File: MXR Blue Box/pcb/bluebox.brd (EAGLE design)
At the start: 59 x 87.8 mm, 20 parts, among them IC2 TL074, J1 POWER_JACK, X1 2510-

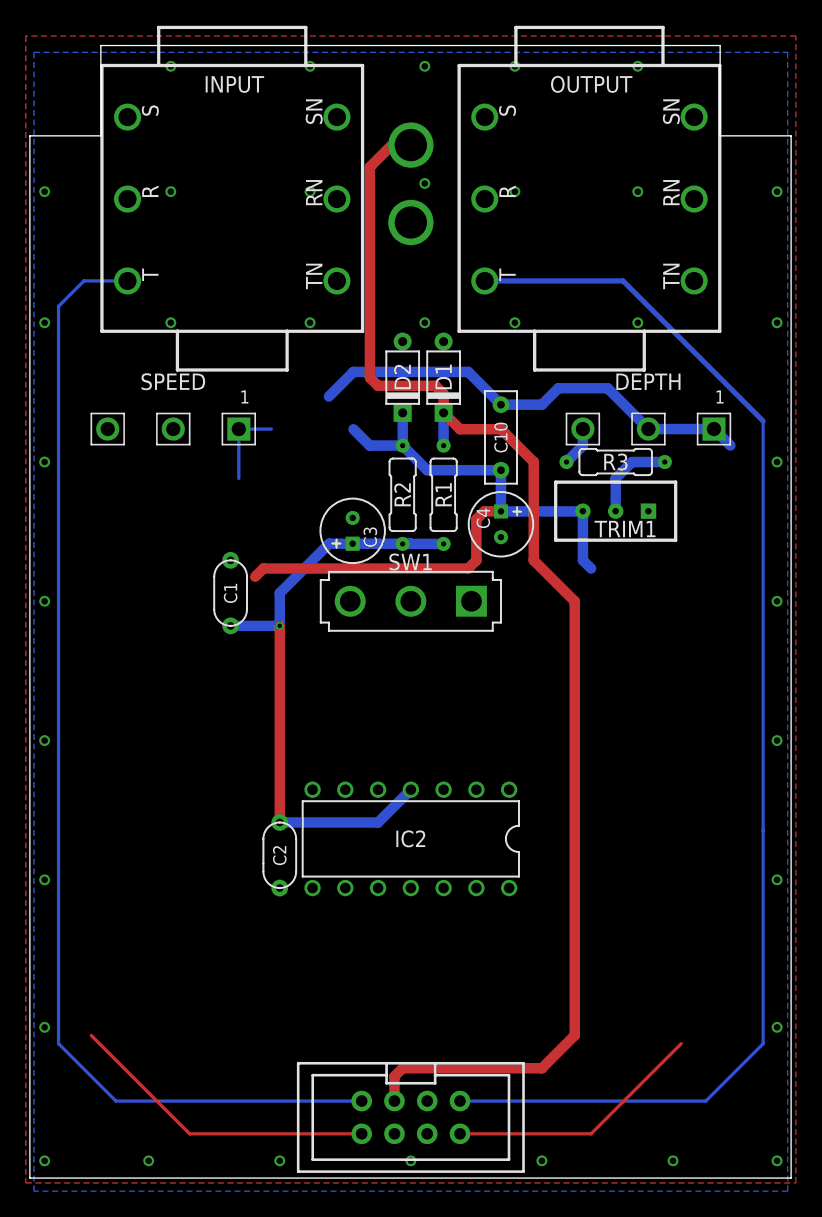
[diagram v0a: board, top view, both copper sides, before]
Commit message: 20171216
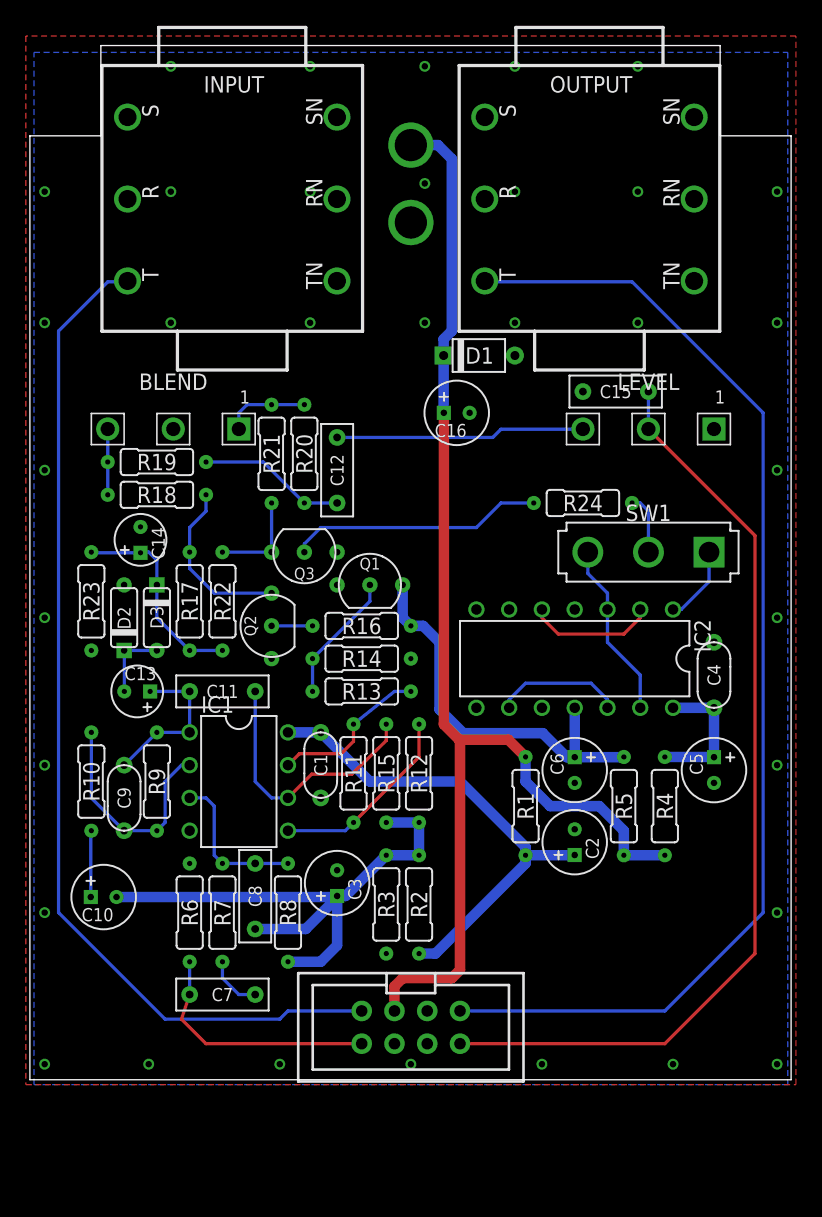
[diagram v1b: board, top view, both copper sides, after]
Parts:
- removed TRIM1: 250k, pedals-potentiometers:RTRIM3296W
- added C11, C12: 47n, pedals-capacitors-film:BOX_SMALL
- added C13, C14: 1u, pedals-capacitors-elec:040_020
- added C15: 6.8n, pedals-capacitors-film:BOX_SMALL
- added C16, C5, C6: 100u, pedals-capacitors-elec:050_020
- added C7: 10n, pedals-capacitors-film:BOX_SMALL
- added C8: 1n, pedals-capacitors-film:BOX_SMALL
- added C9: 330p, pedals-capacitors-film:050X030_025_2
- added D3: 1N914, pedals-diodes:DO35-2
- added IC1: (no value), pedals-integrated circuits:DIL0
- added Q1, Q2, Q3: 2N3904, pedals-transistors:TO92-
- added R10, R7: 150k, pedals-resistors:R0207/3
- added R11, R16, R24, R8: 1M, pedals-resistors:R0207/3
- added R12, R14, R5: 10k, pedals-resistors:R0207/3
- added R13, R15, R17, R18, R19, R20, R21, R22, R23: 56k, pedals-resistors:R0207/3
- added R4: 330, pedals-resistors:R0207/3
- added R6: 2.2M, pedals-resistors:R0207/3
- added R9: 470k, pedals-resistors:R0207/3
- BLEND: value 500kC -> 100kB
- C10: value 47n -> 10u; device pedals-capacitors-film:BOX_SMALL -> pedals-capacitors-elec:050_020
- C2: value 100n -> 100u; device pedals-capacitors-film:050X030_025_2 -> pedals-capacitors-elec:050_020
- C3: value 100u -> 47u
- C4: value 47u -> 100n; device pedals-capacitors-elec:050_020 -> pedals-capacitors-film:050X030_025_2
- D2: value 5.1V -> 1N914; device pedals-diodes:DO41-2 -> pedals-diodes:DO35-2
- IC2: value TL074 -> 4013N
- LEVEL: value 1MB -> 100kB
- R2: value 10k -> 56k
- R3: value 680 -> 56k
- moved C10 47.1 mm to (5.40, 6.92), turned to 0 degrees
- moved R3 38.6 mm to (27.3, 6.35), turned to 90 degrees
- moved R2 31.8 mm to (29.8, 6.35)
- moved D2 28.5 mm to (6.99, 28.6)
- moved C3 27.3 mm to (23.5, 8.00)
- moved R1 25.0 mm to (38.1, 14.0)
- moved C2 22.9 mm to (41.9, 11.2), turned to 90 degrees
- moved C4 20.2 mm to (52.7, 24.1), turned to 90 degrees
- moved IC2 18.9 mm to (41.9, 25.4)
- moved SW1 18.8 mm to (47.6, 33.7)
- moved C1 15.1 mm to (22.2, 17.1), turned to 270 degrees
- moved X1 6.99 mm to (29.2, -3.17)
- moved D1 3.22 mm to (34.5, 48.9), turned to 0 degrees
- renumbered DEPTH to LEVEL, SPEED to BLEND
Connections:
- removed net VA: C10.2, LEVEL.1, LEVEL.2
- new net N$10: IC1.5, R11.1, R12.2
- new net N$11: IC1.7, R11.2, R13.1
- new net N$12: Q1.2, R13.2, R14.2
- new net N$13: Q2.2, R16.2
- new net N$14: Q2.1, R17.1, R18.1
- new net N$15: BLEND.3, R18.2, R19.2
- new net N$16: BLEND.1, R20.2, R21.1
- new net N$17: C12.1, R19.1, R20.1
- new net N$18: C14.+, D3.C, R17.2, R22.2, R23.2
- new net N$20: C13.-, D2.C, D3.A
- new net N$21: C12.2, LEVEL.3
- new net N$22: IC2.13, IC2.3, SW1.3
- new net N$23: IC2.12, IC2.9
- new net N$24: IC2.1, SW1.1
- new net N$25: IC2.2, IC2.5
- new net N$5: C8.1, IC1.3, R7.2, R8.2
- new net N$6: C9.2, IC1.2, R10.2, R9.1
- new net N$7: C11.2, C13.+, C9.1, IC1.1, R9.2
- new net N$8: C10.+, R10.1
- new net N$9: C11.1, IC1.6, R15.2
- new net VC: C4.1, C5.+, IC2.14, R4.2
- new net VD: C6.+, IC2.11, Q1.1, R16.1, R5.2
- net +9V: now also C16.+, R4.1, R5.1
- net GND: now also BLEND.2, C14.-, C15.2, C16.-, C2.-, C4.2, C5.-, C6.-, IC1.4, IC2.10, IC2.4, IC2.6, IC2.7, IC2.8, LEVEL.1, Q1.3, Q2.3, Q3.3, R14.1, R23.1, R3.1, R6.1; no longer C2.2, C4.-, IC2.11, TRIM1.1
- net IN: now also C7.2, R6.2
- net N$1: now also Q3.1, R21.2, R22.1; no longer R3.1, TRIM1.2
- net N$19: now also Q3.2, R24.1; no longer BLEND.1
- net N$27: now also R24.2, SW1.2; no longer BLEND.3
- net N$3: now also C7.1, R7.1; no longer LEVEL.3, R3.2
- net OUT: now also C15.1, LEVEL.2
- net VB: now also C10.-, C3.+, C8.2, R12.1, R15.1, R3.2, R8.1; no longer C10.1, C4.+, D2.C, TRIM1.3
- net VR: now also C2.+, IC1.8; no longer C2.1, C3.+, IC2.4
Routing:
- net OUT: track 20.0 -> 72.7 mm
- net VA: track 35.3 -> 0.00 mm
- net VD: track 0.00 -> 31.0 mm
- net N$9: track 0.00 -> 20.8 mm
- net N$21: track 0.00 -> 19.3 mm
- net N$6: track 0.00 -> 17.7 mm
- net N$18: track 0.00 -> 16.0 mm
- net N$10: track 0.00 -> 15.1 mm
- net N$22: track 0.00 -> 13.7 mm
- net N$14: track 0.00 -> 13.4 mm
- net N$19: track 6.35 -> 19.7 mm
- net N$11: track 0.00 -> 12.5 mm
- net N$7: track 0.00 -> 12.4 mm
- net N$5: track 0.00 -> 12.0 mm
- net N$17: track 0.00 -> 11.5 mm
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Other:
- board size 59 x 87.8 mm -> 59 x 80.2 mm
